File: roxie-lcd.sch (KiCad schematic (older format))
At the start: 7 parts, among them J1 Arduino-NANO-33, J2 VESC, J3 TFT, J4 BUTTON_1, J5 BUTTON_2, J6 BUTTON_3, J7 SD

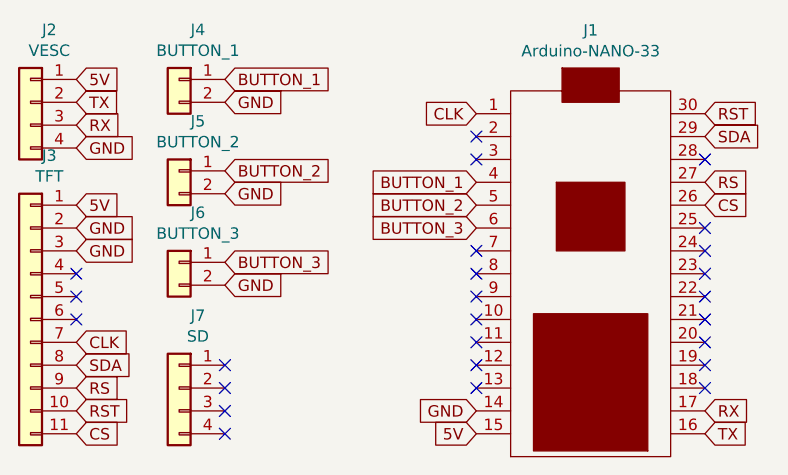
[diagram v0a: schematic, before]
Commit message: first finished version
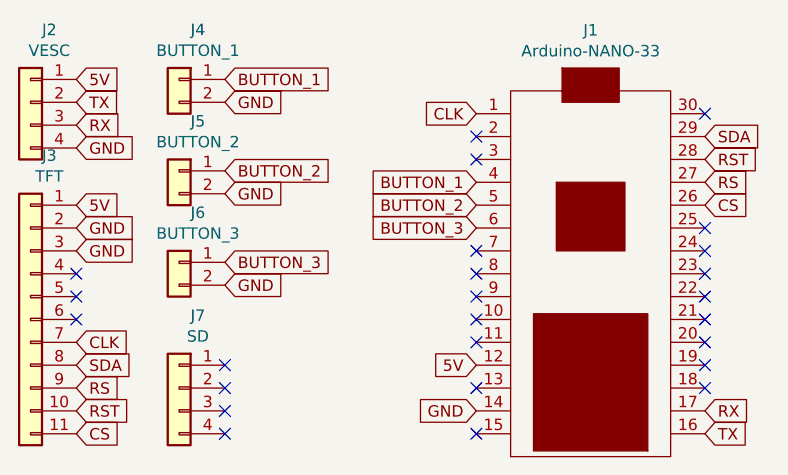
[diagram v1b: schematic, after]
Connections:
- net 5V: now also J1.12; no longer J1.15
- net RST: now also J1.28; no longer J1.30
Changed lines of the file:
@@
 Text GLabel 4500 2550 0    50   Input ~ 0
 GND
-Text GLabel 4500 2650 0    50   Input ~ 0
+Text GLabel 4500 2350 0    50   Input ~ 0
 5V
 $Comp
@@
 Text GLabel 5500 1550 2    50   Input ~ 0
 RS
-Text GLabel 5500 1250 2    50   Input ~ 0
+Text GLabel 5500 1450 2    50   Input ~ 0
 RST
 Text GLabel 5500 1650 2    50   Input ~ 0
@@
 NoConn ~ 4500 2150
 NoConn ~ 4500 2250
-NoConn ~ 4500 2350
+NoConn ~ 4500 2650
 NoConn ~ 4500 2450
 NoConn ~ 5500 2450
@@
 NoConn ~ 5500 1850
 NoConn ~ 5500 1750
-NoConn ~ 5500 1450
+NoConn ~ 5500 1250
 $Comp
 L Connector_Generic:Conn_01x04 J7
